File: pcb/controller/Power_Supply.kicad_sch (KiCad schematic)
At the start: 98 parts, among them J401 JST XH, Q401 DOZ35N06, Q402 2N7002, Q403 2N7002, Q404 2N7002, SW401 SW_SPDT_312, U401 SIC438BED-T1-GE3, U402 TPS259474ARPW, U403 LM74700, U404 LM5166DRCR, U405 BQ25616

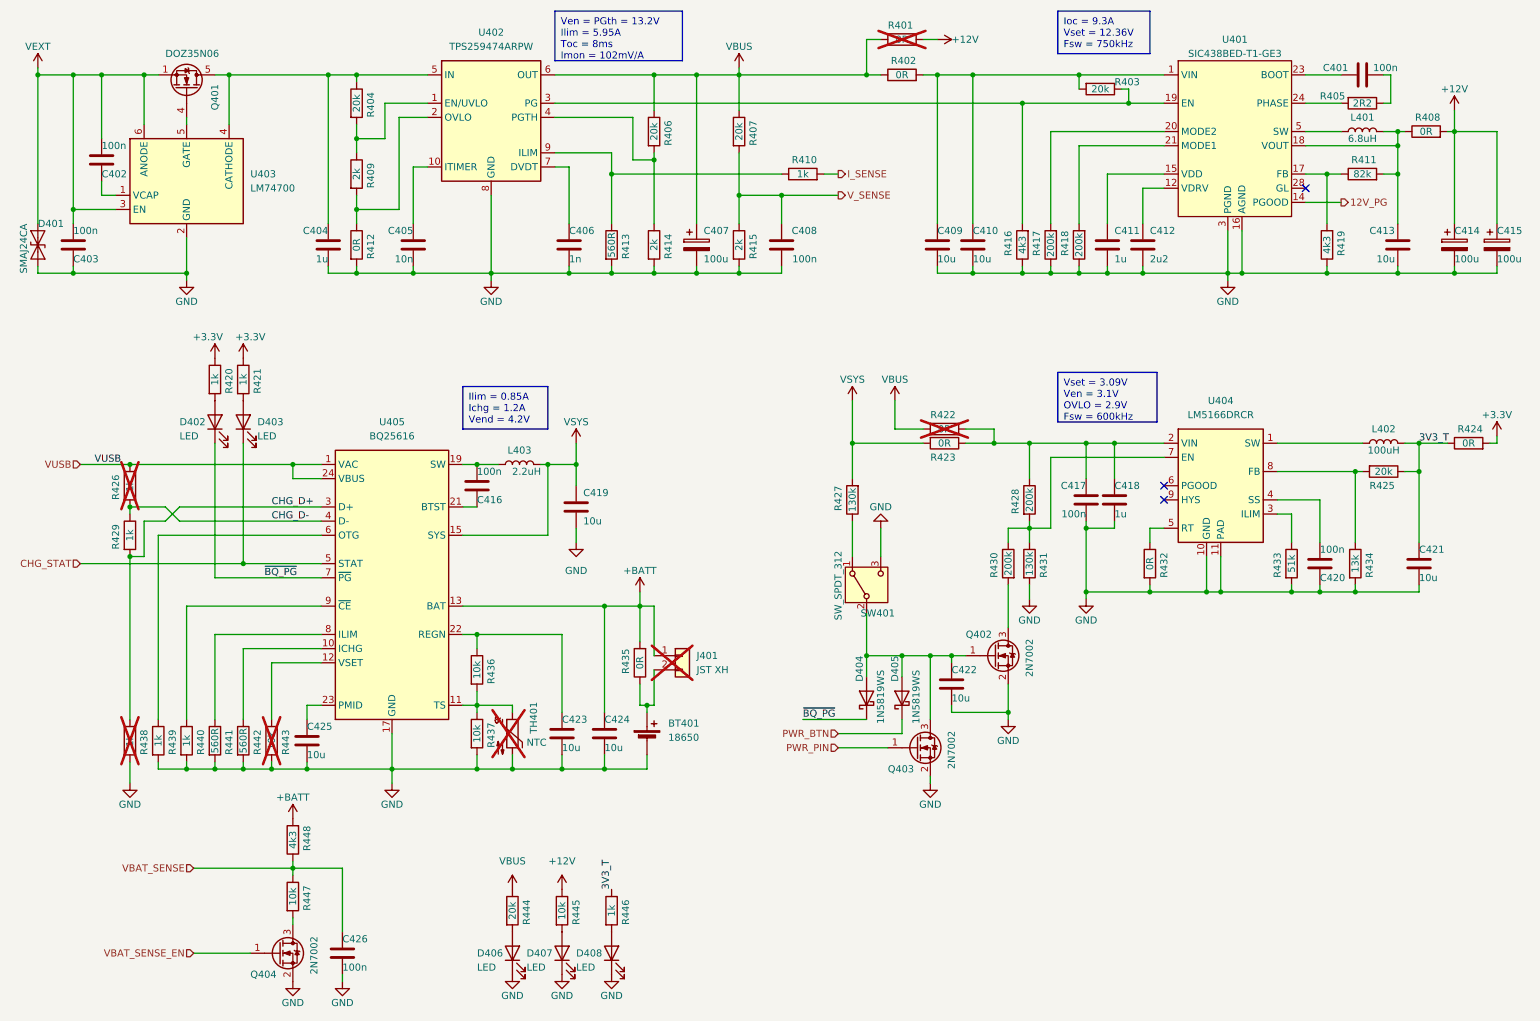
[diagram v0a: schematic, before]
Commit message: Final adjustments and BOM optimization
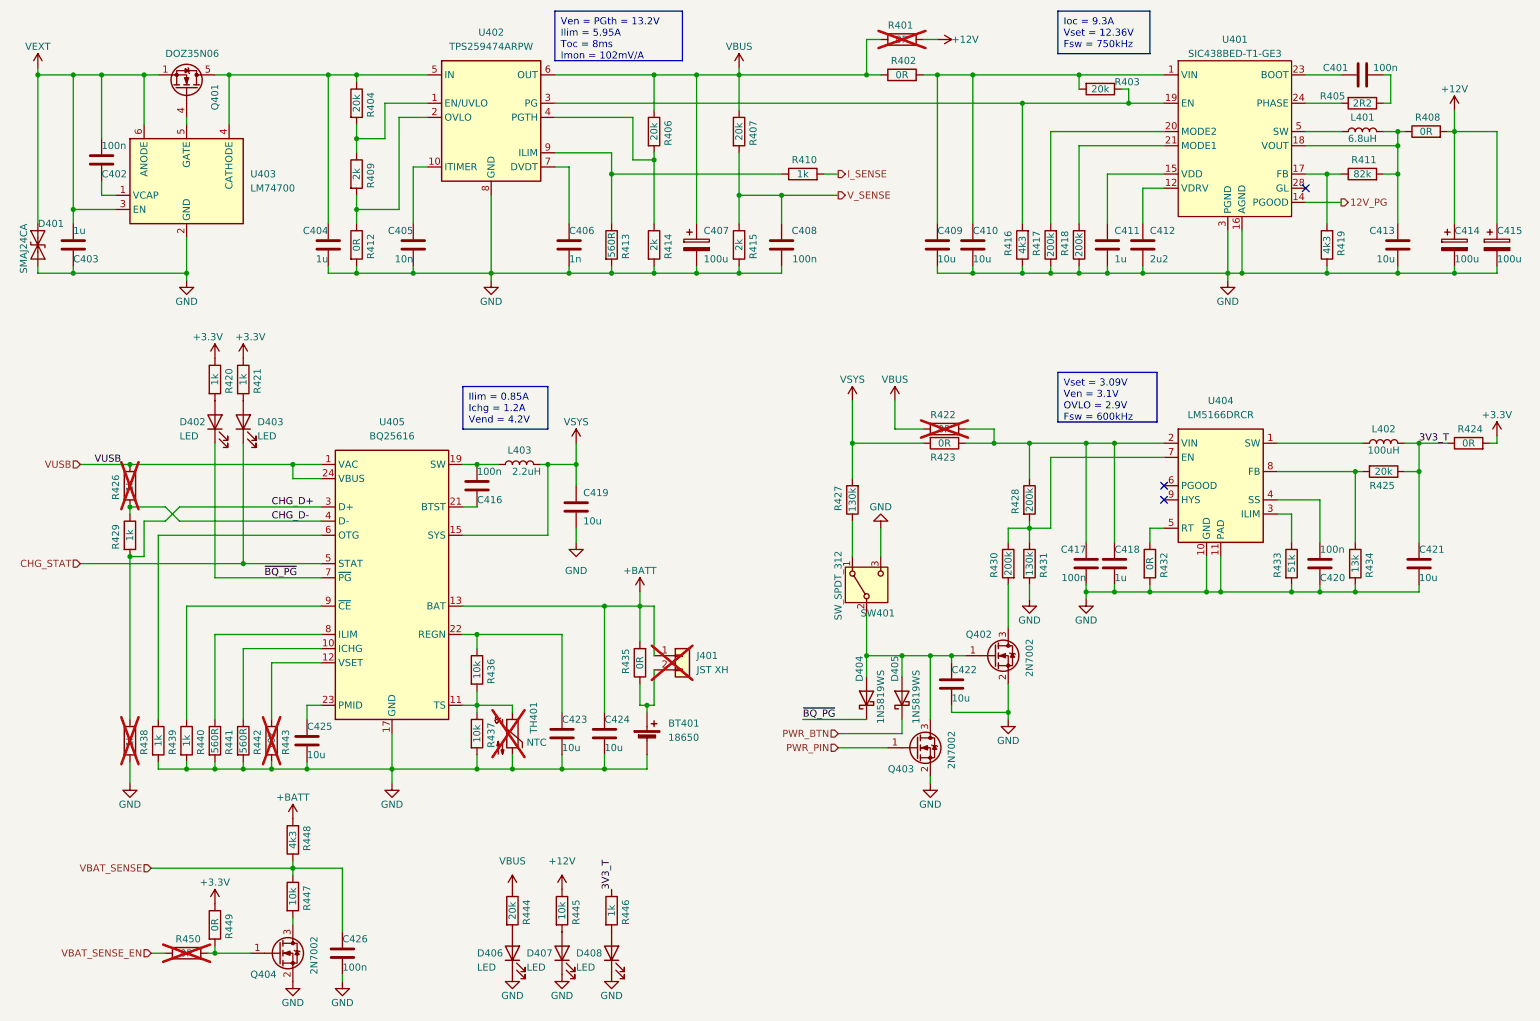
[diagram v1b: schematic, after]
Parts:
- added R449, R450: 0R, Resistor_SMD:R_0402_1005Metric, symbol Device:R
- C403: value 100n -> 1u; footprint Capacitor_SMD:C_0402_1005Metric -> Capacitor_SMD:C_0603_1608Metric; LCSC Part # C307331 -> C15849
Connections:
- net +3.3V: now also R449.1
- net VBAT_SENSE_EN: now also R450.1; no longer Q404.1 (G)
- new net: Q404.1 (G), R449.2, R450.2
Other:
- moved on the sheet: C417, C418
